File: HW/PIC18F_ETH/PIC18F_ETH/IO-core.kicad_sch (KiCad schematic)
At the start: 99 parts, among them J4001 JST,2.54, J4002 JST,2.54, J4003 JST,2.54, J4004 JST,2.54, J4005 JST,2.54, J4006 JST,2.54, J4007 JST,2.54, J4008 JST,2.54, J4009 JST,2.54, J4010 JST,2.54, J4011 JST,2.54, J4012 JST,2.54, J4013 JST,2.54, J4014 JST,2.54, J4015 JST,2.54, J4016 JST,2.54, J4017 JST,2.54, J4018 JST,2.54, J4019 JST,2.54, J4020 JST,2.54, J4021 JST,2.54, J4022 JST,2.54, J4023 JST,2.54, J4024 JST,2.54, J4025 JST,2.54, J4026 JST,2.54, U4001 TLP241B, U4002 TLP241B, U4003 TLP241B, U4004 TLP241B, U4005 TLP241B, U4006 TLP241B, U4007 TLP241B, U4008 TLP241B

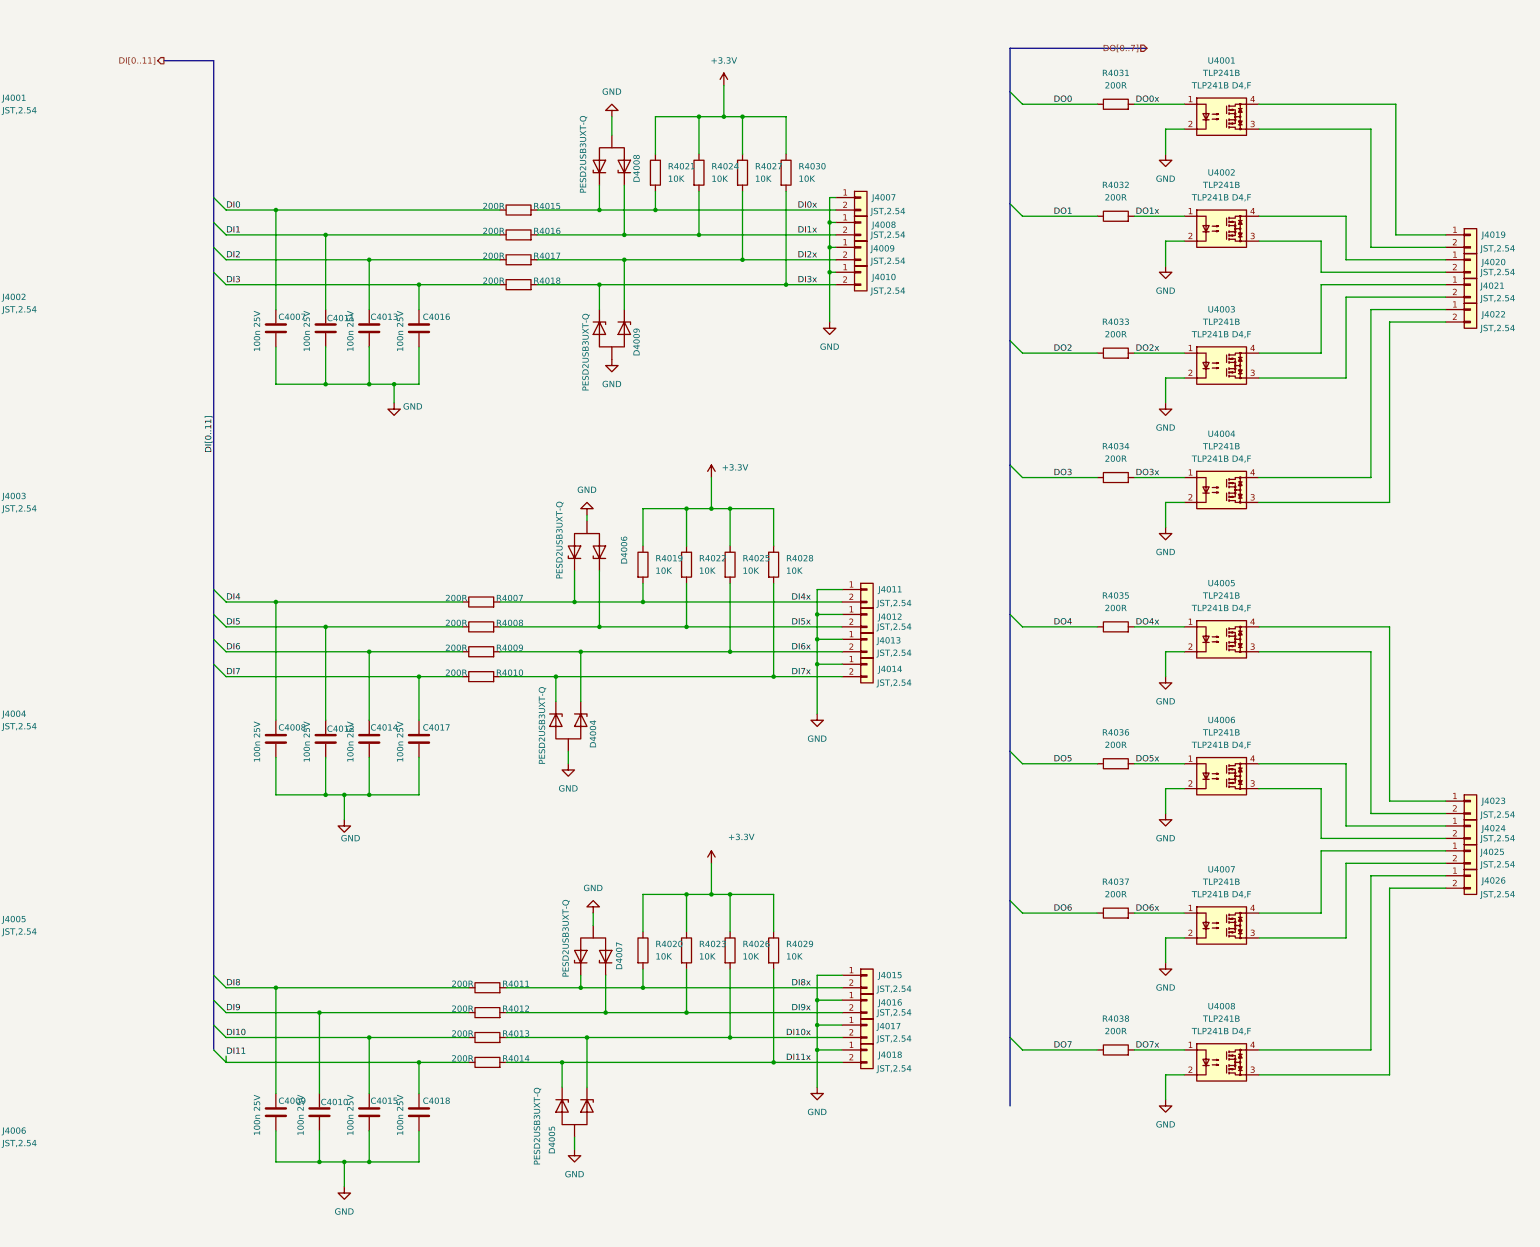
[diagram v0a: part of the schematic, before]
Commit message: .
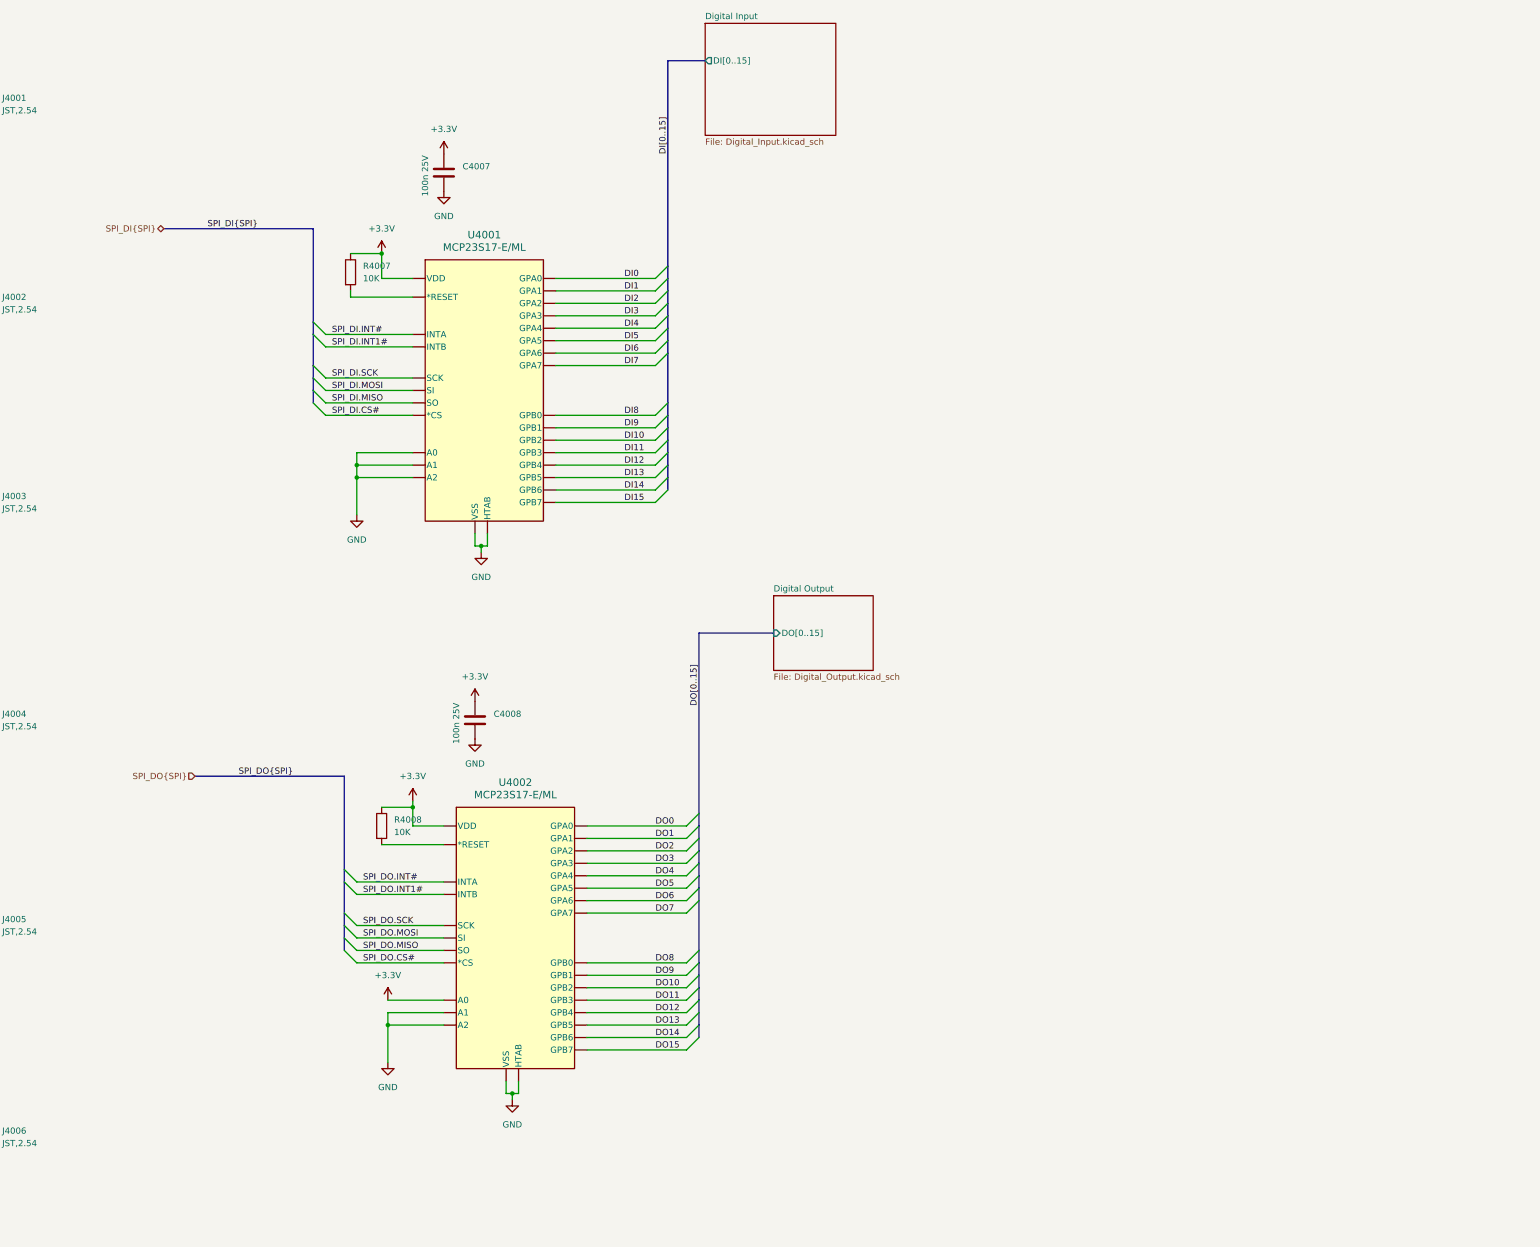
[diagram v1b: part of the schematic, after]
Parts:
- removed C4009, C4010, C4011, C4012, C4013, C4014, C4015, C4016, C4017, C4018: 100n 25V, Capacitor_SMD:C_0603_1608Metric, symbol bt_capacitor:C;M;100n;10p;25V;S;0603
- removed D4004, D4005, D4006, D4007, D4008, D4009: PESD2USB3UXT-Q, Package_TO_SOT_SMD:SOT-23-3, symbol bt_ESD_protection:PESD2USB3UXT-Q
- removed J4007, J4008, J4009, J4010, J4011, J4012, J4013, J4014, J4015, J4016, J4017, J4018, J4019, J4020, J4021, J4022, J4023, J4024, J4025, J4026: JST,2.54, Connector_JST:JST_EH_B2B-EH-A_1x02_P2.50mm_Vertical, symbol bt_connector:M;JST;01x02;2.54
- removed R4007, R4008, R4009, R4010, R4011, R4012, R4013, R4014, R4015, R4016, R4017, R4018, R4031, R4032, R4033, R4034, R4035, R4036, R4037, R4038: 200R, Resistor_SMD:R_0603_1608Metric, symbol bt_resistors:R;G;200R;10P0;S;0603
- removed R4019, R4020, R4021, R4022, R4023, R4024, R4025, R4026, R4027, R4028, R4029, R4030: 10K, Resistor_SMD:R_0603_1608Metric, symbol bt_resistors:R;G;10K;10P0;S;0603
- removed U4001, U4002, U4003, U4004, U4005, U4006, U4007, U4008: TLP241B, Package_SO:SO-4_7.6x3.6mm_P2.54mm, symbol bt_relay:TLP241B-D4-LF1
- added R4007, R4008: 10K, Resistor_SMD:R_0603_1608Metric, symbol bt_resistors:R;G;10K;10P0;S;0603
- added U4001, U4002: MCP23S17-E/ML, bt_footprints:QFN28_6x6MC_MCH, symbol bt_interface:MCP23S17-E_ML
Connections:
- net +3.3V: now also C4007.1, C4008.1, R4007.1, R4008.1, U4001.5 (VDD), U4002.11 (A0), U4002.5 (VDD)
- net DI0: now also U4001.17 (GPA0); no longer C4007.1
- net DI1: now also U4001.18 (GPA1)
- net DI10: now also U4001.27 (GPB2)
- net DI11: now also U4001.28 (GPB3)
- net DI2: now also U4001.19 (GPA2)
- net DI3: now also U4001.20 (GPA3)
- net DI4: now also U4001.21 (GPA4); no longer C4008.1
- net DI5: now also U4001.22 (GPA5)
- net DI6: now also U4001.23 (GPA6)
- net DI7: now also U4001.24 (GPA7)
- net DI8: now also U4001.25 (GPB0)
- net DI9: now also U4001.26 (GPB1)
- net DO0: now also U4002.17 (GPA0)
- net DO1: now also U4002.18 (GPA1)
- net DO2: now also U4002.19 (GPA2)
- net DO3: now also U4002.20 (GPA3)
- net DO4: now also U4002.21 (GPA4)
- net DO5: now also U4002.22 (GPA5)
- net DO6: now also U4002.23 (GPA6)
- net DO7: now also U4002.24 (GPA7)
- net GND: now also U4001.11 (A0), U4001.12 (A1), U4001.13 (A2), U4001.29 (HTAB), U4001.6 (VSS), U4002.12 (A1), U4002.13 (A2), U4002.29 (HTAB), U4002.6 (VSS)
- new net: R4007.2, U4001.14 (*RESET)
- new net: R4008.2, U4002.14 (*RESET)
- new net DI12: U4001.1 (GPB4)
- new net DI13: U4001.2 (GPB5)
- new net DI14: U4001.3 (GPB6)
- new net DI15: U4001.4 (GPB7)
- new net DO10: U4002.27 (GPB2)
- new net DO11: U4002.28 (GPB3)
- new net DO12: U4002.1 (GPB4)
- new net DO13: U4002.2 (GPB5)
- new net DO14: U4002.3 (GPB6)
- new net DO15: U4002.4 (GPB7)
- new net DO8: U4002.25 (GPB0)
- new net DO9: U4002.26 (GPB1)
- new net SPI_DI.CS#: U4001.7 (*CS)
- new net SPI_DI.INT#: U4001.16 (INTA)
- new net SPI_DI.INT1#: U4001.15 (INTB)
- new net SPI_DI.MISO: U4001.10 (SO)
- new net SPI_DI.MOSI: U4001.9 (SI)
- new net SPI_DI.SCK: U4001.8 (SCK)
- new net SPI_DO.CS#: U4002.7 (*CS)
- new net SPI_DO.INT#: U4002.16 (INTA)
- new net SPI_DO.INT1#: U4002.15 (INTB)
- new net SPI_DO.MISO: U4002.10 (SO)
- new net SPI_DO.MOSI: U4002.9 (SI)
- new net SPI_DO.SCK: U4002.8 (SCK)
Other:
- added sheet Digital Input (Digital_Input.kicad_sch)
- added sheet Digital Output (Digital_Output.kicad_sch)
